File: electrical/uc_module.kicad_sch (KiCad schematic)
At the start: 8 parts, among them J6 Conn_01x06_Pin, SW2 SW_SPST, U1 ATtiny84A-PU

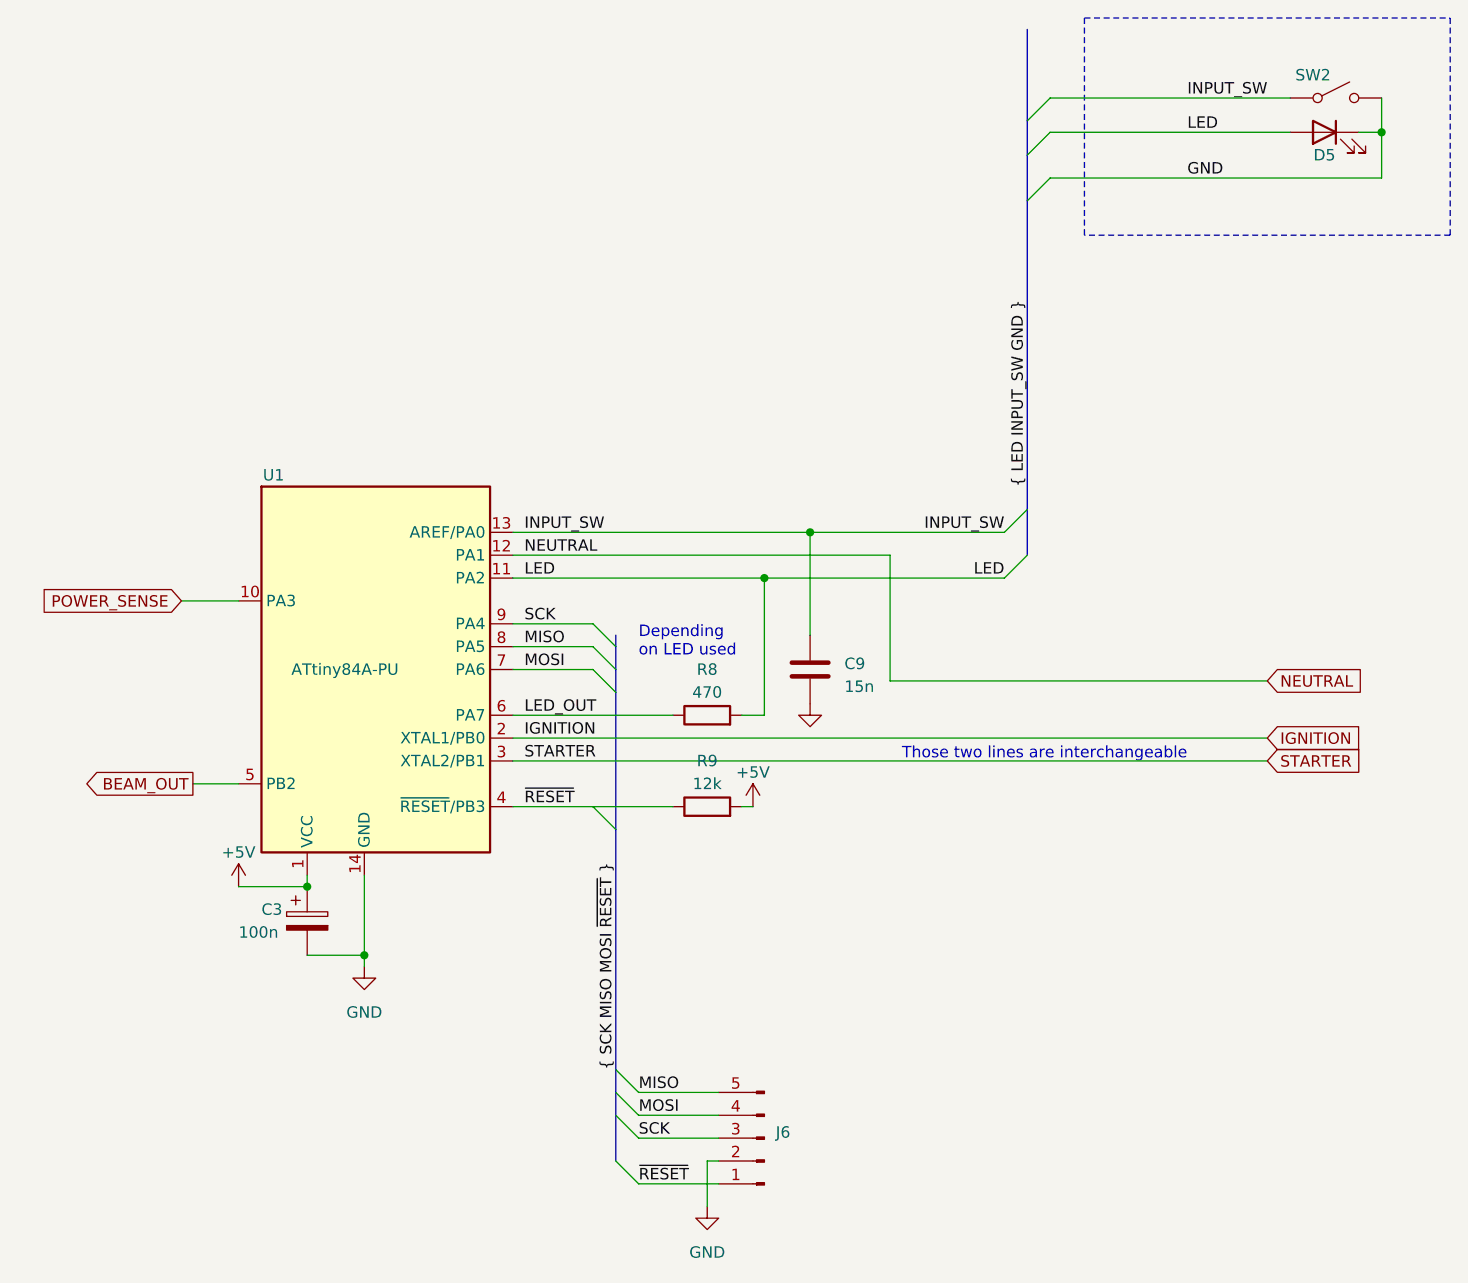
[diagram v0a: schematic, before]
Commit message: Work in progress
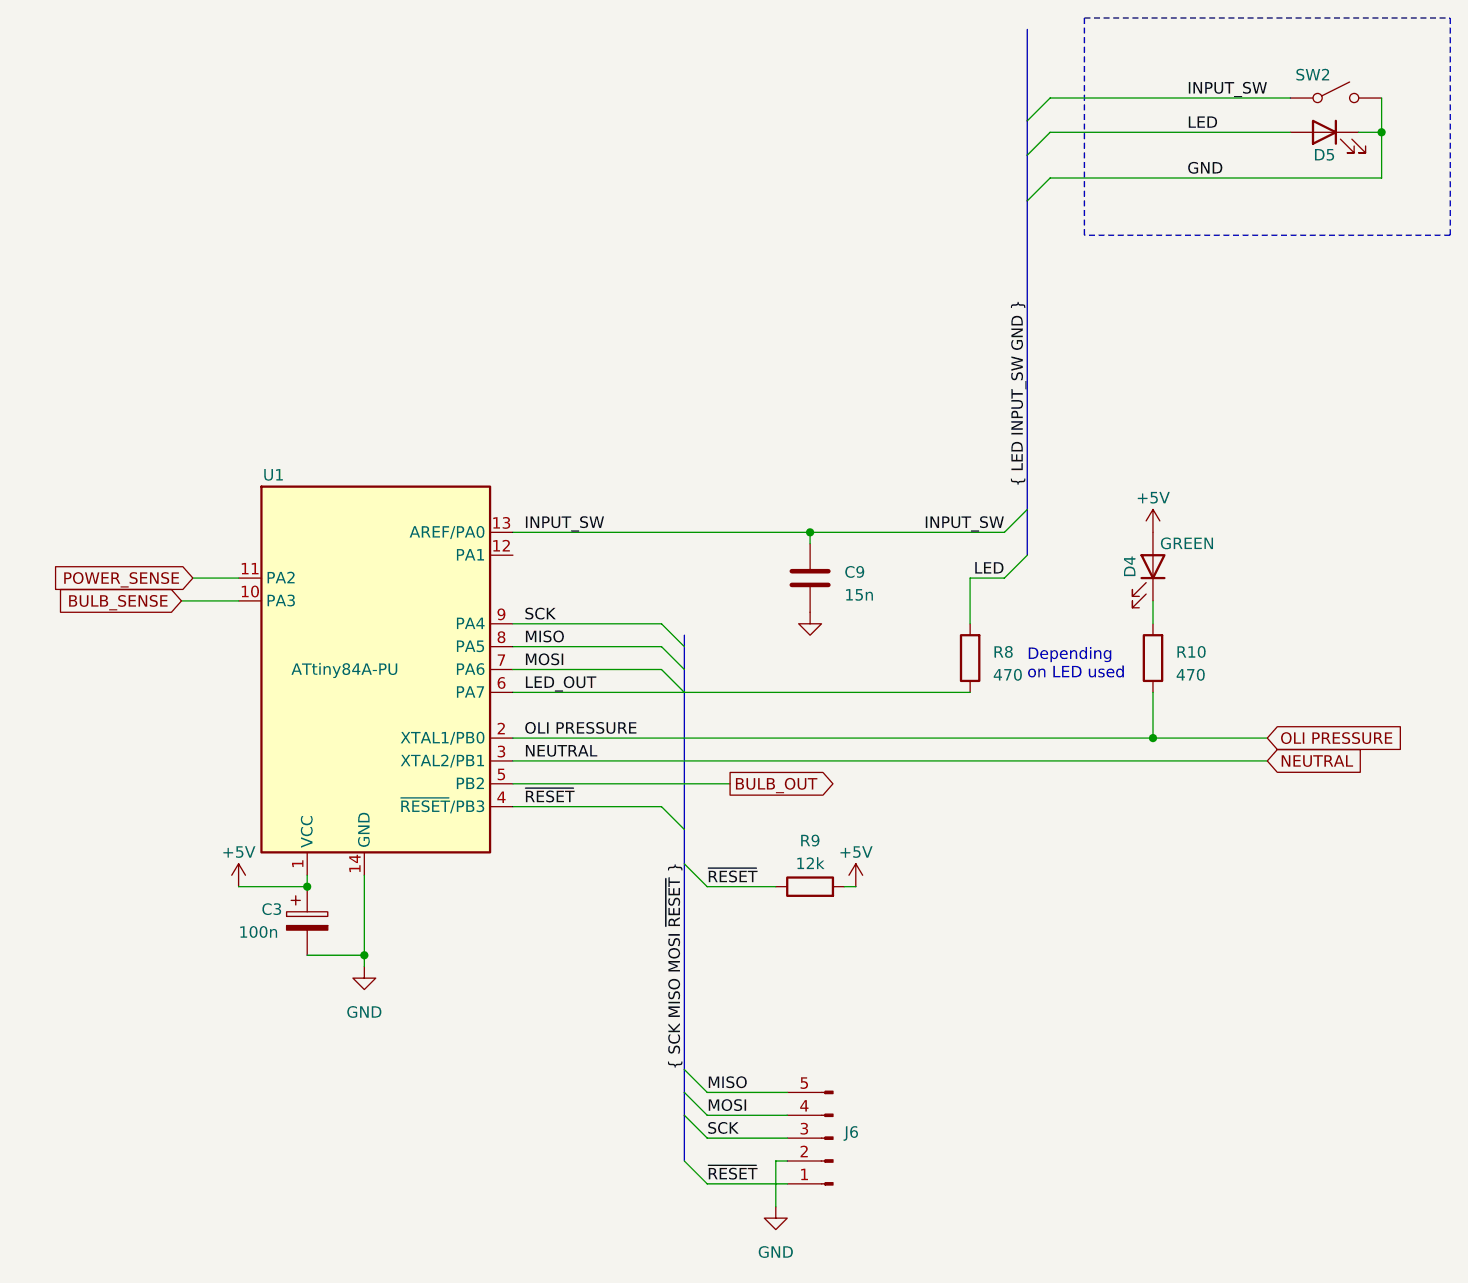
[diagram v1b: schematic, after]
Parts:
- added D4: GREEN, symbol Device:LED
- added R10: 470, symbol Device:R
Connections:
- net STARTER is gone; now on net NEUTRAL: U1.3 (XTAL2/PB1)
- net +5V: now also D4.2 (A)
- net LED: no longer U1.11 (PA2)
- net NEUTRAL: no longer U1.12 (PA1)
- net POWER_SENSE: now also U1.11 (PA2); no longer U1.10 (PA3)
- net BEAM_OUT renamed BULB_OUT
- net IGNITION renamed OLI PRESSURE
- net OLI PRESSURE: now also R10.1
- new net: D4.1 (K), R10.2
- new net BULB_SENSE: U1.10 (PA3)
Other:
- note removed: "Those two lines are interchangeable"
- moved on the sheet: C9, J6, R8, R9
